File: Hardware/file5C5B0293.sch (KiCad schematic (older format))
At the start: 27 parts, among them J16 Conn_01x06_Male, J17 Conn_ARM_JTAG_SWD_10, J24 Digital_Connector, J25 CV_Connector, J26 Pot_Connector, J27 Attenuverter_Connector, U13 STM32F303RBTx

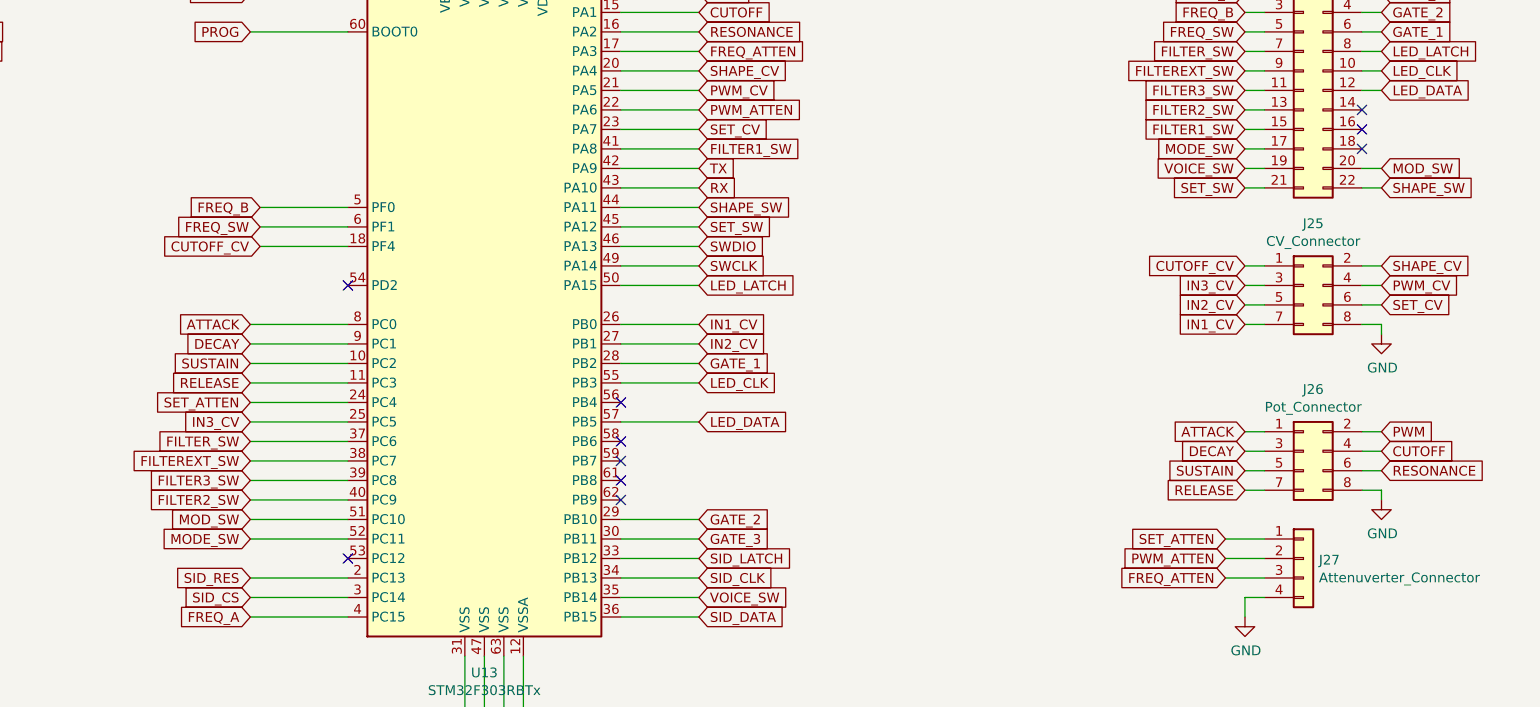
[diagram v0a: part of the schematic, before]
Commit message: Fixes #10
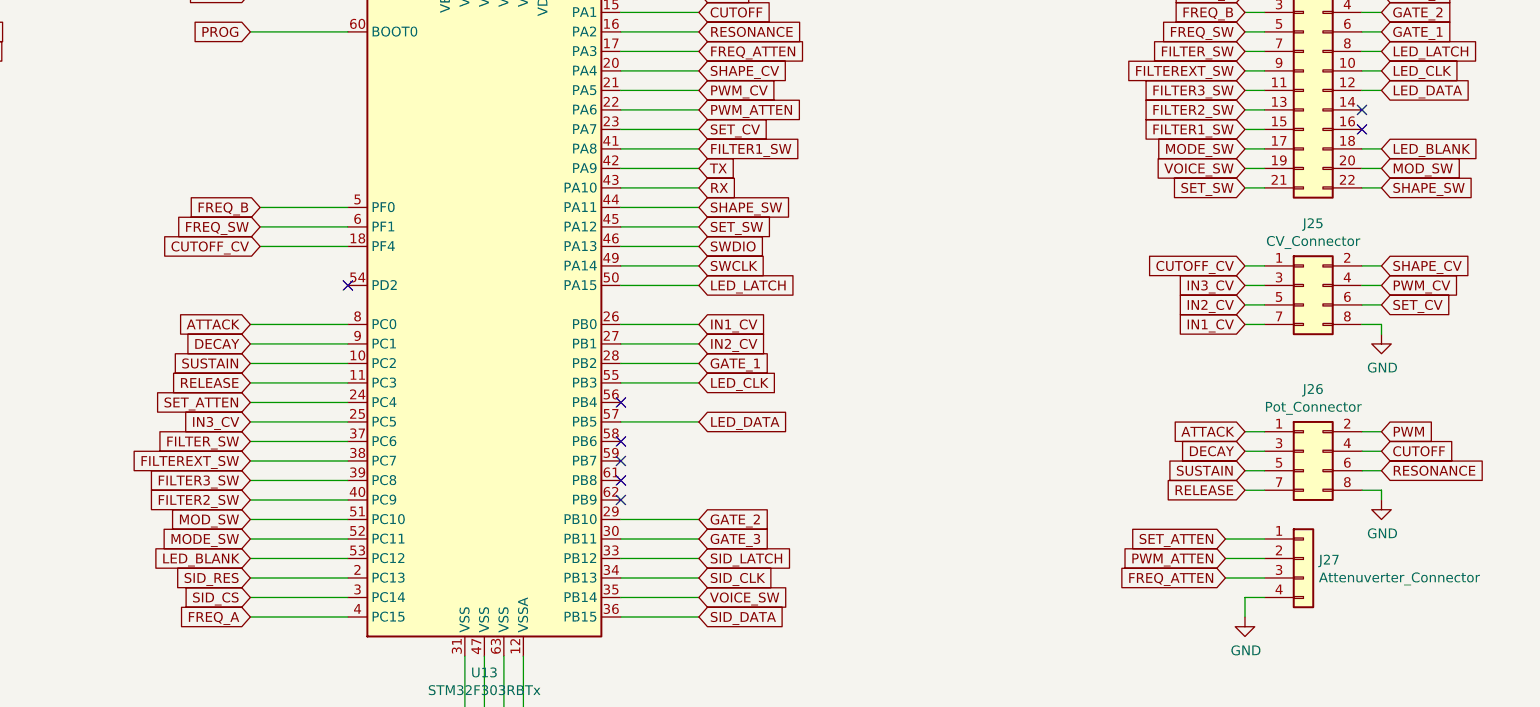
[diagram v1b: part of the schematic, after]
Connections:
- net LED_BLANK: now reaches U13.53 (PC12)
- net LED_BLANK: now also J24.18 (Pin_18)
- no-connect marks 16 -> 14
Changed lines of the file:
@@
 	6100 2850 6500 2850
 NoConn ~ 4700 3450
-NoConn ~ 4700 4850
 NoConn ~ 6100 4550
 NoConn ~ 6100 4450
@@
 NoConn ~ 9900 2550
 NoConn ~ 9900 2650
-NoConn ~ 9900 2750
+Text GLabel 4200 4850 0    50   Input ~ 0
+LED_BLANK
+Wire Wire Line
+	4200 4850 4700 4850
+Text GLabel 10000 2750 2    50   Input ~ 0
+LED_BLANK
+Wire Wire Line
+	10000 2750 9900 2750
 $EndSCHEMATC
